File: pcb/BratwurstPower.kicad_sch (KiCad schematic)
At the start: 32 parts, among them J1 BarrelJack, J2 Raspi, J3 USB1in, J4 USB1out, J5 I2C, J6 I2C, J7 USB2in, J8 USB2out, J9 EXT, Q1 AO3401A, U1 PCA9557PW

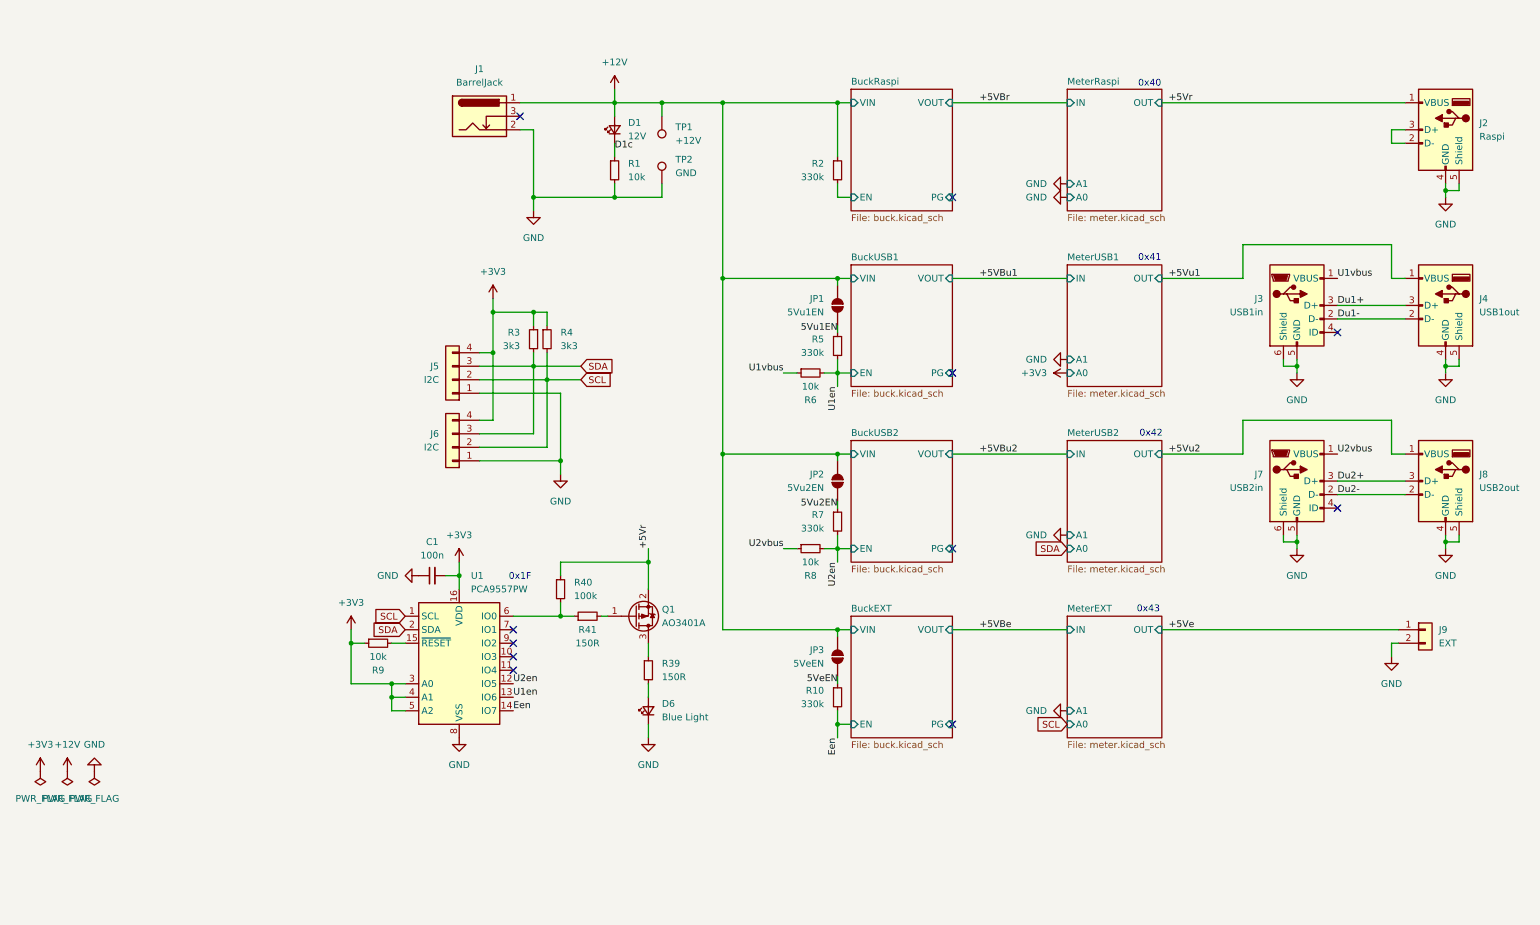
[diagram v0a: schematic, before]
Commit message: feat: featuritis
added too much stuff...
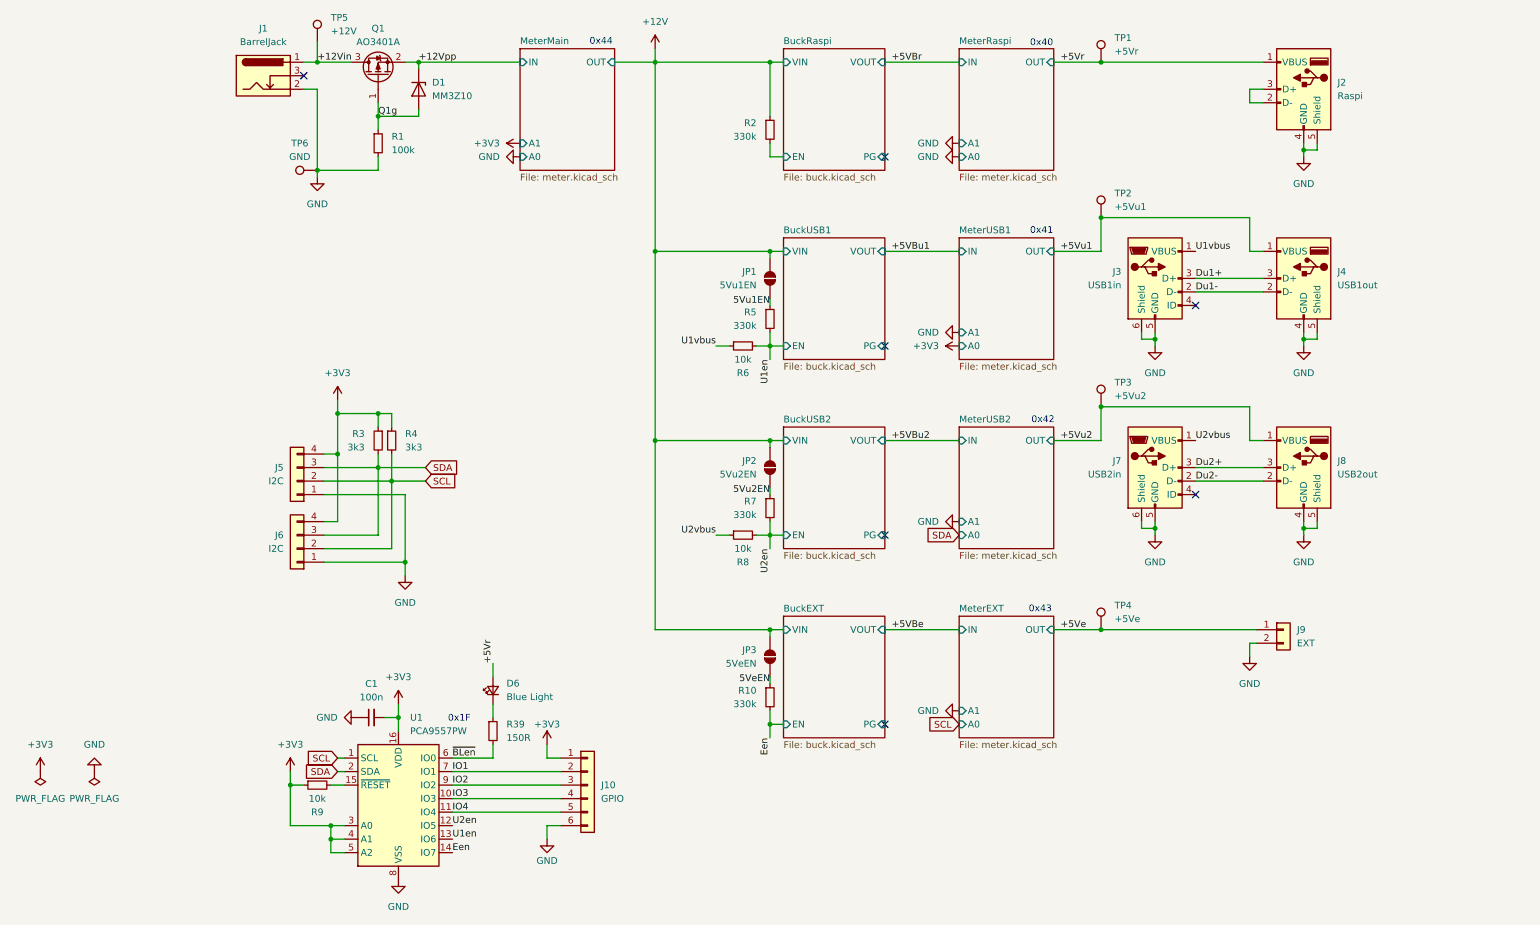
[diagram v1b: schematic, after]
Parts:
- removed D1: 12V, LED_SMD:LED_0603_1608Metric, symbol Device:LED_Small
- removed R40: 100k, Resistor_SMD:R_0402_1005Metric, symbol Device:R_Small
- removed R41: 150R, Resistor_SMD:R_0402_1005Metric, symbol Device:R_Small
- added D1: MM3Z10, Diode_SMD:D_SOD-323F, symbol Diode:MM3Zxx
- added J10: GPIO, Connector_PinHeader_2.54mm:PinHeader_1x06_P2.54mm_Vertical, symbol Connector_Generic:Conn_01x06
- added TP3: +5Vu2, TestPoint:TestPoint_THTPad_D1.0mm_Drill0.5mm, symbol Connector:TestPoint
- added TP4: +5Ve, TestPoint:TestPoint_THTPad_D1.0mm_Drill0.5mm, symbol Connector:TestPoint
- added TP5: +12V, TestPoint:TestPoint_THTPad_D2.0mm_Drill1.0mm, symbol Connector:TestPoint
- added TP6: GND, TestPoint:TestPoint_THTPad_D2.0mm_Drill1.0mm, symbol Connector:TestPoint
- R1: value 10k -> 100k; LCSC C25744 -> (none)
- TP1: value +12V -> +5Vr; footprint TestPoint:TestPoint_Pad_D1.5mm -> TestPoint:TestPoint_THTPad_D1.0mm_Drill0.5mm; now in the parts list
- TP2: value GND -> +5Vu1; footprint TestPoint:TestPoint_Pad_D1.5mm -> TestPoint:TestPoint_THTPad_D1.0mm_Drill0.5mm; now in the parts list
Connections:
- net D1c is gone; now on net Q1g: R1.1
- net +12V: no longer J1.1, TP1.1
- net +3V3: now also J10.1 (Pin_1)
- net +5Ve: now also TP4.1
- net +5Vr: now also D6.2 (A), TP1.1; no longer Q1.2 (S)
- net +5Vu1: now also TP2.1
- net +5Vu2: now also TP3.1
- net GND: now also J10.6 (Pin_6), TP6.1; no longer D6.1 (K), TP2.1
- net Q1g: now reaches Q1.1 (G)
- net Q1g: now also D1.2 (A)
- net at R39.1: now also D6.1 (K); no longer Q1.3 (D)
- net IO3: now reaches U1.10 (IO3)
- net IO3: now also J10.4 (Pin_4)
- net IO4: now reaches U1.11 (IO4)
- net IO4: now also J10.5 (Pin_5)
- net ~{BLen}: now reaches U1.6 (IO0)
- net ~{BLen}: now also R39.2
- net IO1: now reaches U1.7 (IO1)
- net IO1: now also J10.2 (Pin_2)
- net IO2: now reaches U1.9 (IO2)
- net IO2: now also J10.3 (Pin_3)
- new net +12Vin: J1.1, Q1.3 (D), TP5.1
- new net +12Vpp: D1.1 (K), Q1.2 (S)
- no-connect marks 11 -> 7
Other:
- added sheet MeterMain (meter.kicad_sch)
- note added: "0x44"
- moved on the sheet: C1, D6, J1, J2, J3, J4, J5, J6, J7, J8, J9, JP1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

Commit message: chore: cleanup
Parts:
- D1: LCSC (none) -> C19077459
- Q1: LCSC (none) -> C15127
- R1: LCSC (none) -> C25741
- R39: LCSC (none) -> C25082
- TP1, TP2, TP3, TP4, TP5, TP6: now left out of the parts list
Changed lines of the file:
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@@
 			)
 		)
+		(property "LCSC" "C19077459"
+			(at 50.8 34.29 0)
+			(effects
+				(font
+					(size 1.27 1.27)
+				)
+				(hide yes)
+			)
+		)
 		(pin "1"
 		)
@@
 		(unit 1)
 		(exclude_from_sim no)
-		(in_bom yes)
+		(in_bom no)
 		(on_board yes)
 		(dnp no)
@@
 		(unit 1)
 		(exclude_from_sim no)
-		(in_bom yes)
+		(in_bom no)
 		(on_board yes)
 		(dnp no)
@@
 		(unit 1)
 		(exclude_from_sim no)
-		(in_bom yes)
+		(in_bom no)
 		(on_board yes)
 		(dnp no)
@@
 		(unit 1)
 		(exclude_from_sim no)
-		(in_bom yes)
+		(in_bom no)
 		(on_board yes)
 		(dnp no)
@@
 			)
 		)
+		(property "LCSC" "C25082"
+			(at 64.77 154.94 0)
+			(effects
+				(font
+					(size 1.27 1.27)
+				)
+				(hide yes)
+			)
+		)
 		(pin "2"
 		)
@@
 		(unit 1)
 		(exclude_from_sim no)
-		(in_bom yes)
+		(in_bom no)
 		(on_board yes)
 		(dnp no)
@@
 			)
 		)
+		(property "LCSC" "C25741"
+			(at 43.18 44.45 0)
+			(effects
+				(font
+					(size 1.27 1.27)
+				)
+				(hide yes)
+			)
+		)
 		(pin "1"
 		)
@@
 			)
 		)
+		(property "LCSC" "C15127"
+			(at 43.18 31.75 0)
+			(effects
+				(font
+					(size 1.27 1.27)
+				)
+				(hide yes)
+			)
+		)
 		(pin "2"
 		)
@@
 		(unit 1)
 		(exclude_from_sim no)
-		(in_bom yes)
+		(in_bom no)
 		(on_board yes)
 		(dnp no)
